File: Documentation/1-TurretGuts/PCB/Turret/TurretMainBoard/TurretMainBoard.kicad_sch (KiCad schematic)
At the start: 82 parts, among them J1 USB_C_Receptacle, J2 SMA-RP, J3 Trigger Conn, J4 Joystick Conn, J5 LED, J6 BatteryLED, J7 2PolSwitch, J8 18650 BATTERY, J9 Spare Conn, Q1 FS8205A, Q2 AO3401A, U2 TP4056-42-ESOP8, U3 ATmega32U4-A, U4 nRF24L01P, U5 RFX2401C, U6 AMS1117, U8 DW01A, U9 MT3608, Y2 16 MHz, Y3 16MHz

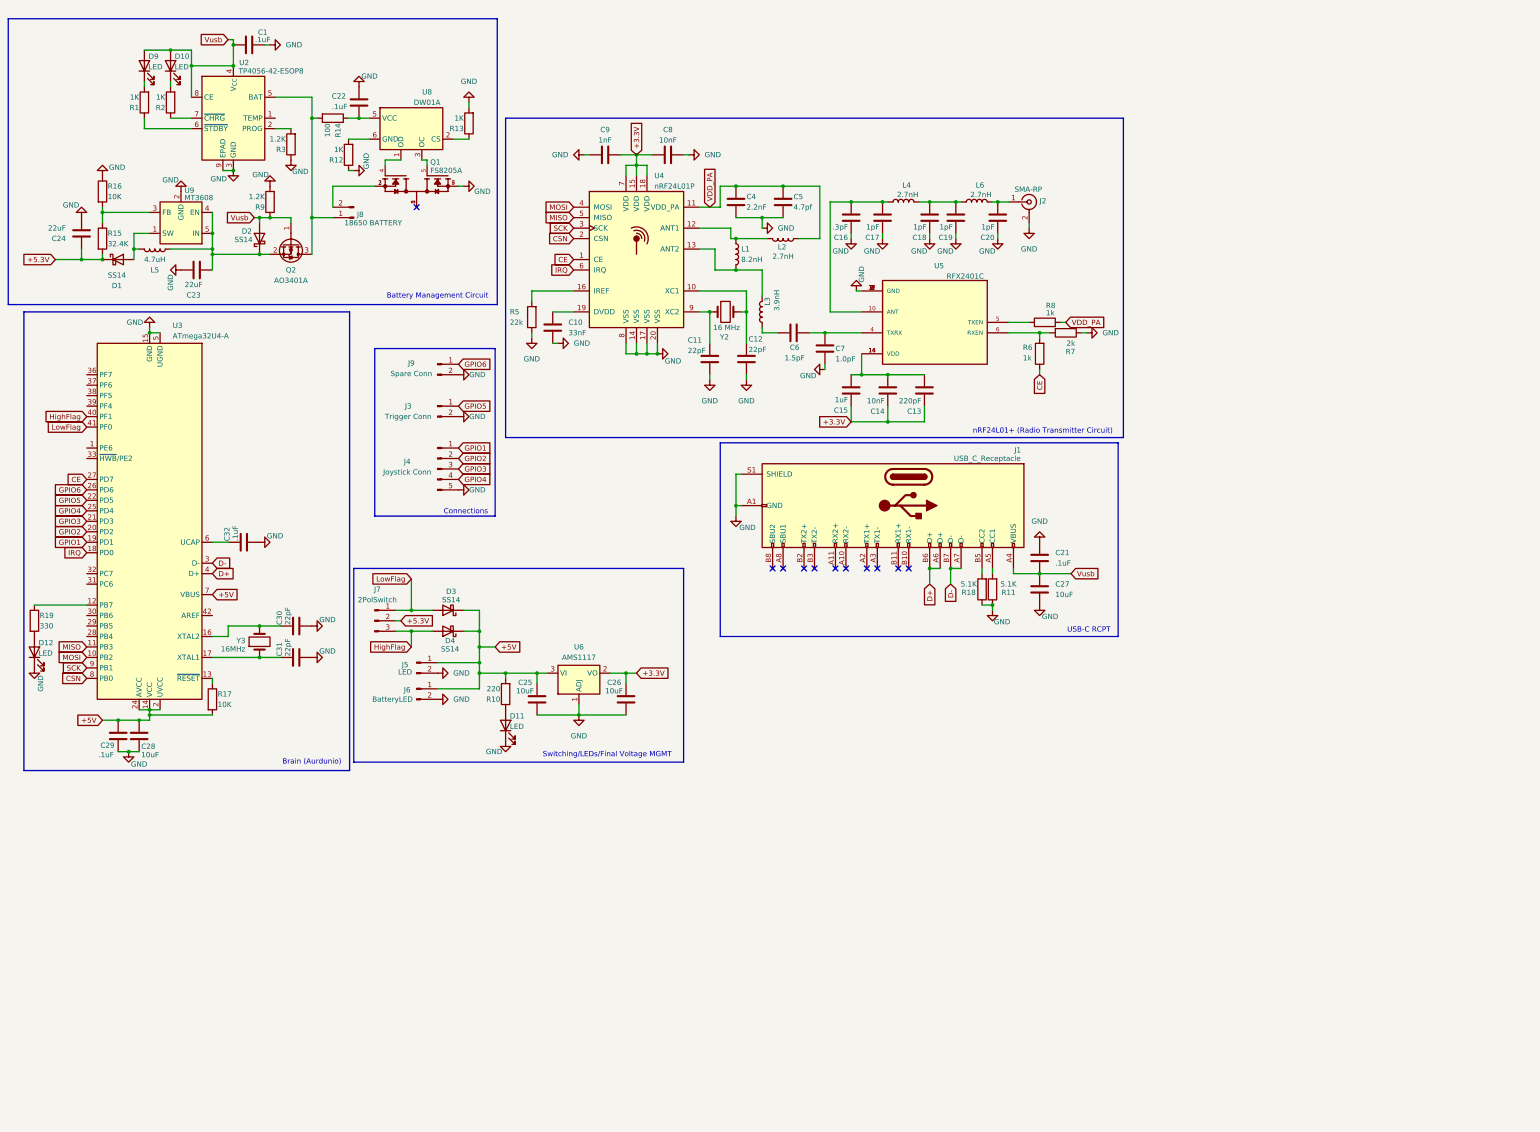
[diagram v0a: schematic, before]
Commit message: sync with main
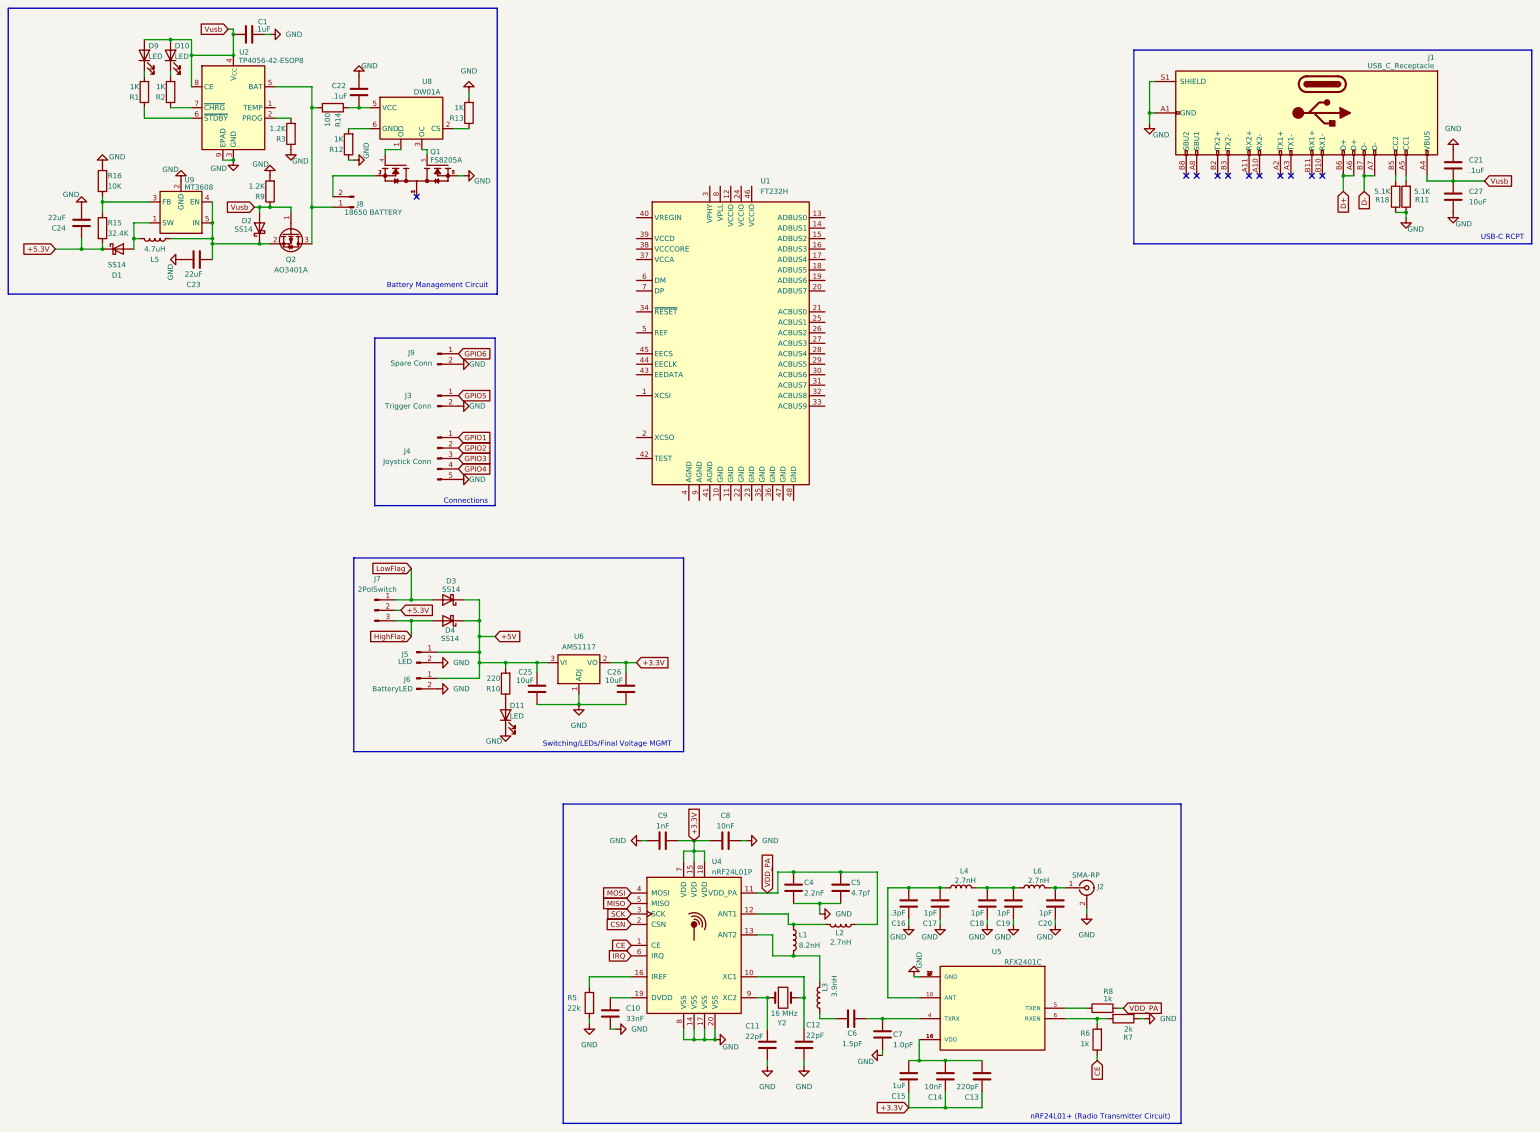
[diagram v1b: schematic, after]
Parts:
- removed C28: 10uF, symbol Device:C
- removed C29, C32: .1uF, symbol Device:C
- removed C30, C31: 22pF, symbol Device:C
- removed D12: LED, symbol Device:LED
- removed R17: 10K, symbol Device:R
- removed R19: 330, symbol Device:R
- removed U3: ATmega32U4-A, Package_QFP:TQFP-44_10x10mm_P0.8mm, symbol MCU_Microchip_ATmega:ATmega32U4-A
- removed Y3: 16MHz, symbol Device:Crystal
- added U1: FT232H, symbol Interface_USB:FT232H
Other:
- note removed: "Brain (Aurdunio)"
- moved on the sheet: C1, C10, C11, C12, C13, C14, C15, C16, C17, C18, C19, C20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
